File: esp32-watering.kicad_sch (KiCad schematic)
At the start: 17 parts, among them J1 5V, J2 12V, J3 Water Level, K1 Pump Control, K2 Zone 1, K3 Zone 2, K4 Zone 3, Q1 PN2222A, Q2 PN2222A, Q3 PN2222A, Q4 PN2222A, U1 esp32-wemos-d1-mini

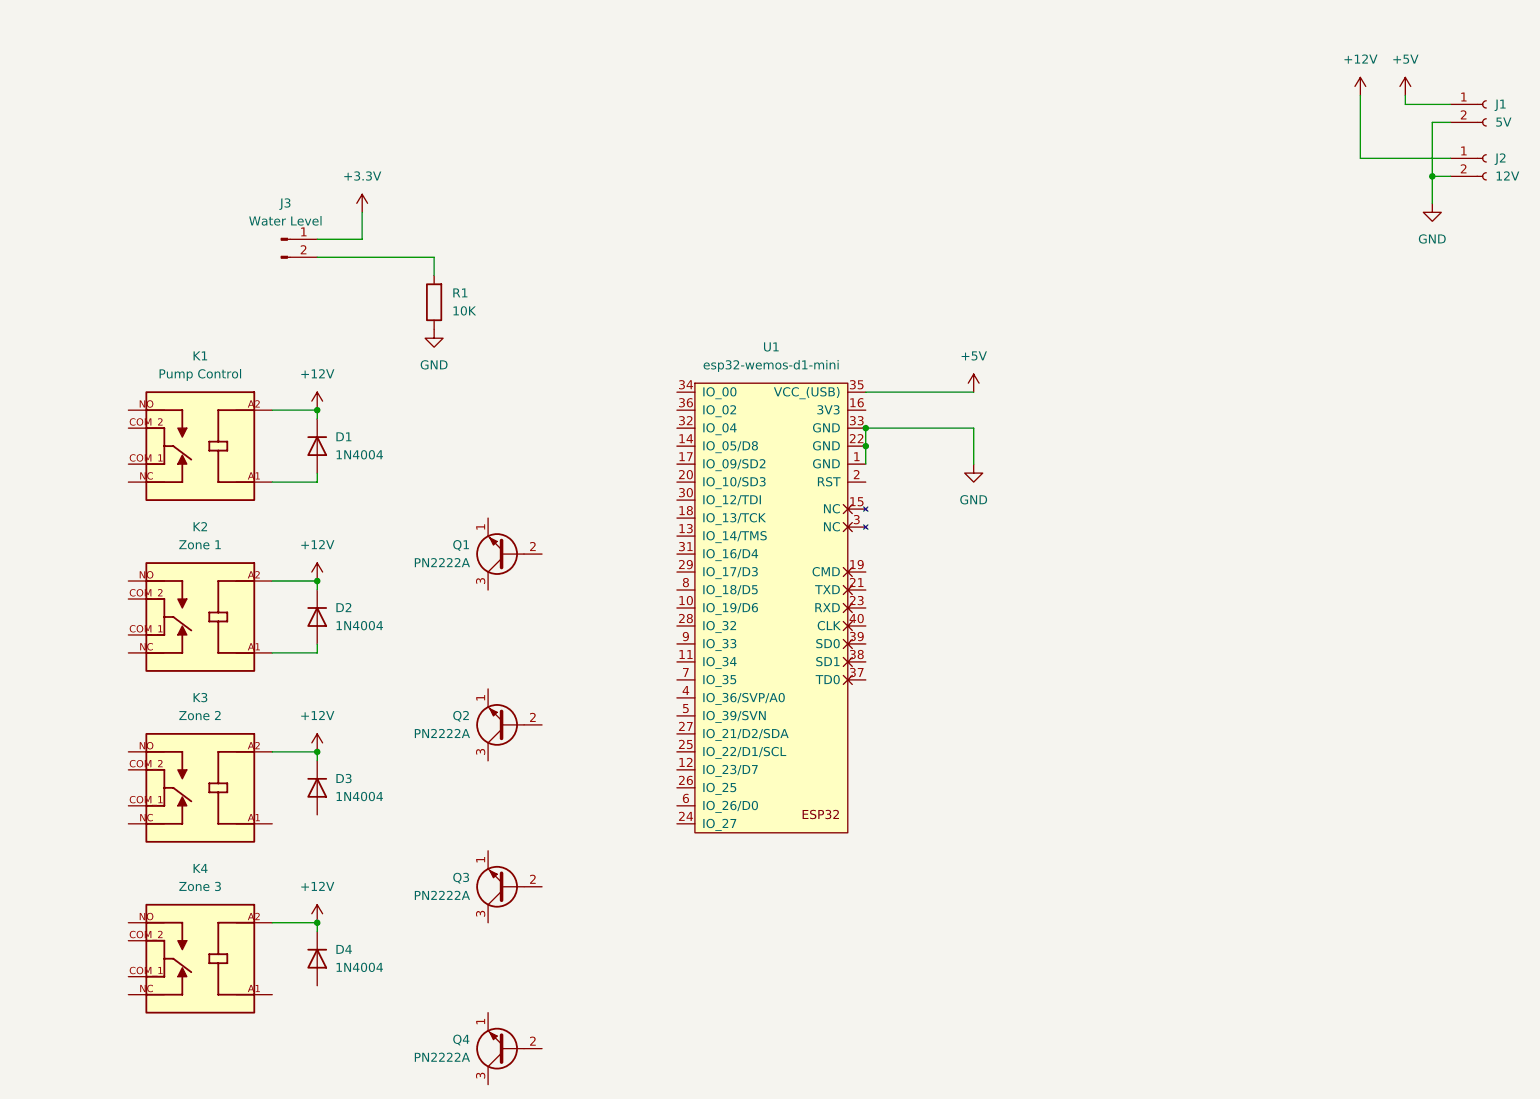
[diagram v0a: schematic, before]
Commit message: First pass of schematic. Three zones.
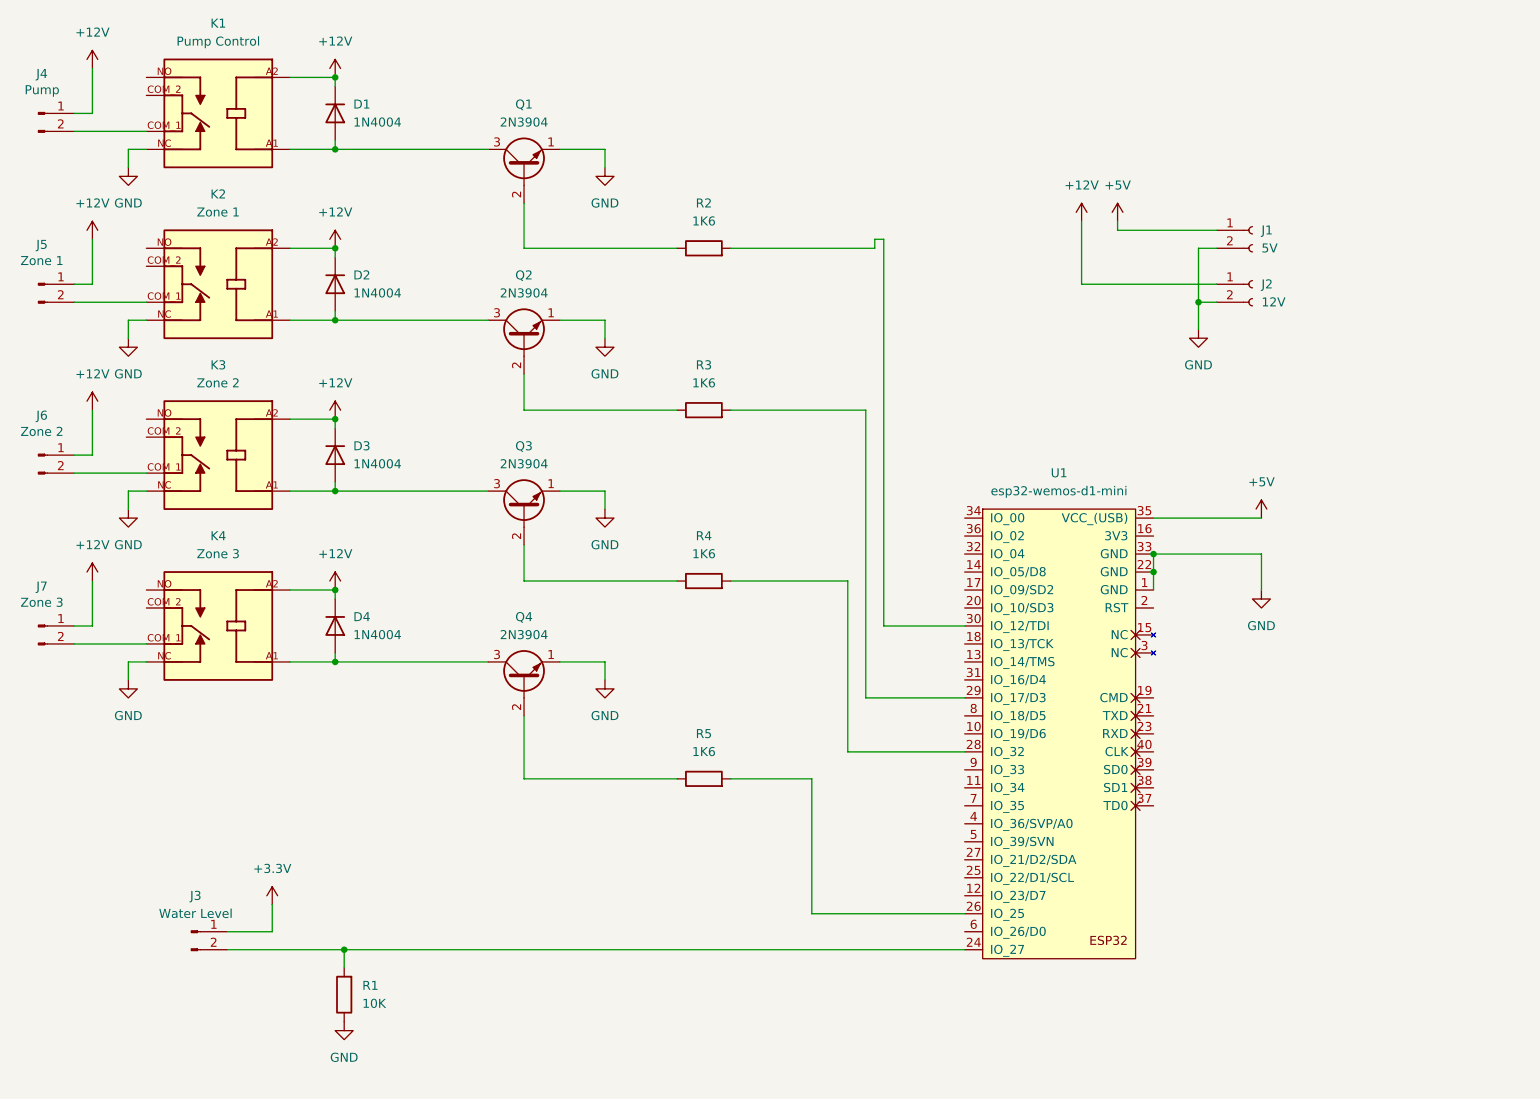
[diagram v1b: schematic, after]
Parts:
- added J4: Pump, Connector_JST:JST_XH_B2B-XH-A_1x02_P2.50mm_Vertical, symbol Connector:Conn_01x02_Pin
- added J5: Zone 1, Connector_JST:JST_XH_B2B-XH-A_1x02_P2.50mm_Vertical, symbol Connector:Conn_01x02_Pin
- added J6: Zone 2, Connector_JST:JST_XH_B2B-XH-A_1x02_P2.50mm_Vertical, symbol Connector:Conn_01x02_Pin
- added J7: Zone 3, Connector_JST:JST_XH_B2B-XH-A_1x02_P2.50mm_Vertical, symbol Connector:Conn_01x02_Pin
- added R2, R3, R4, R5: 1K6, symbol Device:R
- Q1, Q2, Q3, Q4: value PN2222A -> 2N3904; footprint Package_TO_SOT_THT:TO-92L_HandSolder -> Package_TO_SOT_THT:TO-92_Inline; symbol Transistor_BJT:PN2222A -> Transistor_BJT:2N3904
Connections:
- net +12V: now also J4.1 (Pin_1), J5.1 (Pin_1), J6.1 (Pin_1), J7.1 (Pin_1)
- net GND: now also K1.NC, K2.NC, K3.NC, K4.NC, Q1.1 (E), Q2.1 (E), Q3.1 (E), Q4.1 (E)
- net at D2.2 (A), K2.A1: now also Q2.3 (C)
- net at D3.2 (A): now also K3.A1, Q3.3 (C)
- net at Q1.2 (B): now also R2.1
- net at Q1.3 (C): now also D1.2 (A), K1.A1
- net at Q3.2 (B): now also R4.1
- net at D4.2 (A): now also K4.A1, Q4.3 (C)
- net at K1.COM_1: now also J4.2 (Pin_2)
- net at K3.COM_1: now also J6.2 (Pin_2)
- net at Q4.2 (B): now also R5.1
- net at J3.2 (Pin_2), R1.2: now also U1.24 (IO_27)
- net at Q2.2 (B): now also R3.1
- net at K2.COM_1: now also J5.2 (Pin_2)
- net at K4.COM_1: now also J7.2 (Pin_2)
- net at U1.26 (IO_25): now also R5.2
- net at U1.28 (IO_32): now also R4.2
- net at U1.29 (IO_17/D3): now also R3.2
- net at U1.30 (IO_12/TDI): now also R2.2
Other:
- moved on the sheet: D1, D2, D3, D4, J1, J2, J3, K1, K2, K3, K4, Q1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

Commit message: Start layout
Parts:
- J1, J2: footprint Connector_JST:JST_XH_S2B-XH-A-1_1x02_P2.50mm_Horizontal -> Connector_JST:JST_XH_B2B-XH-A_1x02_P2.50mm_Vertical
- R1, R2, R3, R4, R5: footprint (none) -> Resistor_THT:R_Axial_DIN0204_L3.6mm_D1.6mm_P7.62mm_Horizontal
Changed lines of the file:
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@@
 			)
 		)
-		(property "Footprint" ""
+		(property "Footprint" "Resistor_THT:R_Axial_DIN0204_L3.6mm_D1.6mm_P7.62mm_Horizontal"
 			(at 132.08 74.168 90)
 			(effects
@@
 			)
 		)
-		(property "Footprint" ""
+		(property "Footprint" "Resistor_THT:R_Axial_DIN0204_L3.6mm_D1.6mm_P7.62mm_Horizontal"
 			(at 132.08 51.308 90)
 			(effects
@@
 			)
 		)
-		(property "Footprint" "Connector_JST:JST_XH_S2B-XH-A-1_1x02_P2.50mm_Horizontal"
+		(property "Footprint" "Connector_JST:JST_XH_B2B-XH-A_1x02_P2.50mm_Vertical"
 			(at 209.55 46.99 0)
 			(effects
@@
 			)
 		)
-		(property "Footprint" ""
+		(property "Footprint" "Resistor_THT:R_Axial_DIN0204_L3.6mm_D1.6mm_P7.62mm_Horizontal"
 			(at 132.08 98.298 90)
 			(effects
@@
 			)
 		)
-		(property "Footprint" ""
+		(property "Footprint" "Resistor_THT:R_Axial_DIN0204_L3.6mm_D1.6mm_P7.62mm_Horizontal"
 			(at 132.08 126.238 90)
 			(effects
@@
 			)
 		)
-		(property "Footprint" "Connector_JST:JST_XH_S2B-XH-A-1_1x02_P2.50mm_Horizontal"
+		(property "Footprint" "Connector_JST:JST_XH_B2B-XH-A_1x02_P2.50mm_Vertical"
 			(at 209.55 54.61 0)
 			(effects
@@
 			)
 		)
-		(property "Footprint" ""
+		(property "Footprint" "Resistor_THT:R_Axial_DIN0204_L3.6mm_D1.6mm_P7.62mm_Horizontal"
 			(at 83.058 154.94 90)
 			(effects
